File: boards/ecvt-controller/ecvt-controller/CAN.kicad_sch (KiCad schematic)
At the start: 19 parts, among them SW1 SW_SPST, SW2 SW_SPST, U1 TJA1051T-3, U3 MCP2515-xSO, U5 ACT45B-101-2P-TL003, U6 PESD2CAN,215, Y1 Crystal

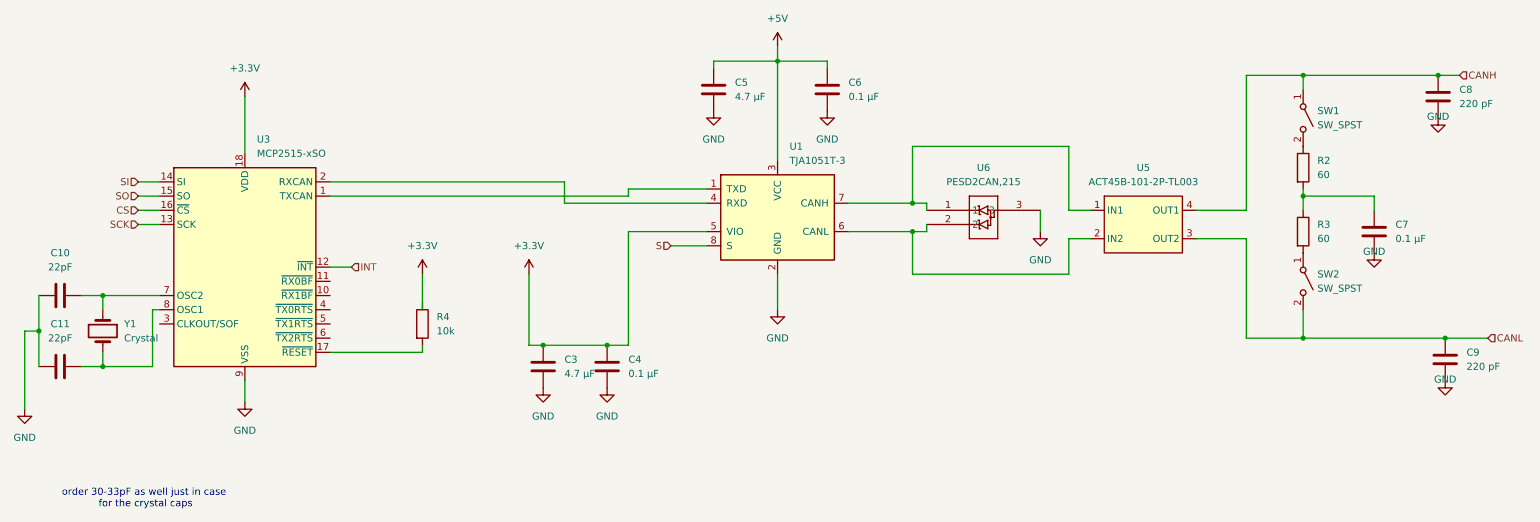
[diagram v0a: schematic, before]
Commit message: components done. RAHHHHH
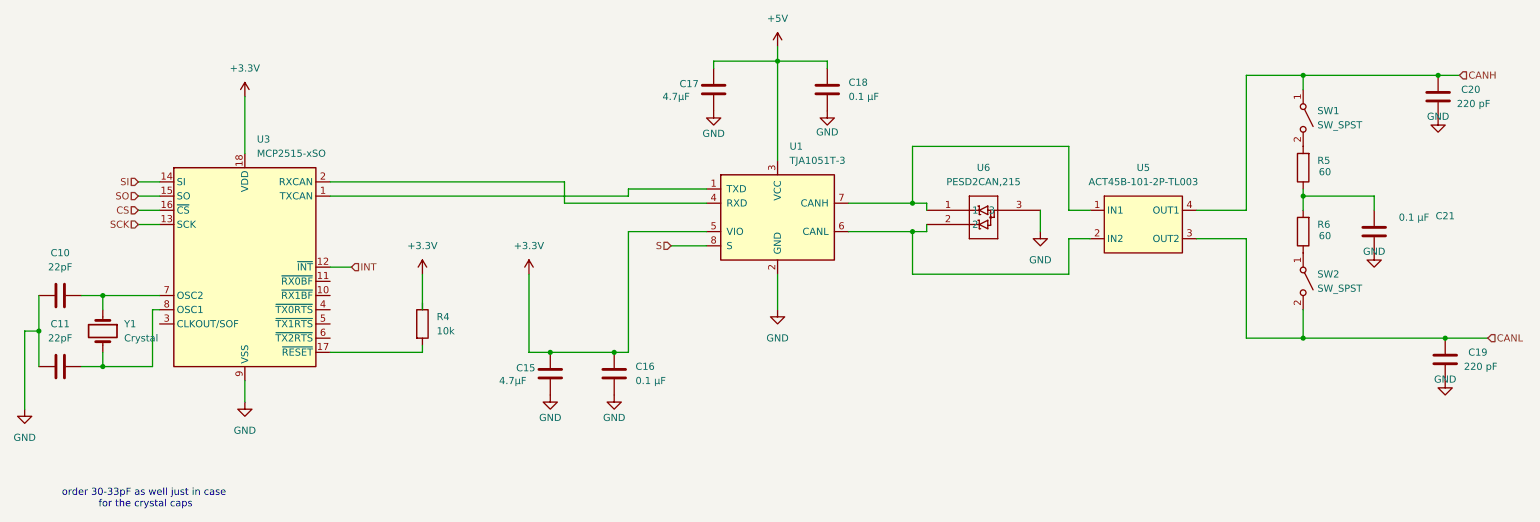
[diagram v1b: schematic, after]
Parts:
- removed C3, C5: 4.7 µF, symbol Device:C
- removed C4, C6, C7: 0.1 µF, symbol Device:C
- removed C8, C9: 220 pF, symbol Device:C
- removed R2, R3: 60, symbol Device:R
- added C15, C17: 4.7µF, Capacitor_SMD:C_0603_1608Metric_Pad1.08x0.95mm_HandSolder, symbol Device:C
- added C16, C18, C21: 0.1 µF, Capacitor_SMD:C_0603_1608Metric_Pad1.08x0.95mm_HandSolder, symbol Device:C
- added C19, C20: 220 pF, Capacitor_SMD:C_0603_1608Metric_Pad1.08x0.95mm_HandSolder, symbol Device:C
- added R5, R6: 60, Resistor_SMD:R_1206_3216Metric_Pad1.30x1.75mm_HandSolder, symbol Device:R
- C10, C11: footprint (none) -> Capacitor_SMD:C_0805_2012Metric_Pad1.18x1.45mm_HandSolder
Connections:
- net +3.3V: now also C15.1, C16.1
- net +5V: now also C17.1, C18.1
- net CANH: now also C20.1
- net CANL: now also C19.1
- net GND: now also C15.2, C16.2, C17.2, C18.2, C19.2, C20.2, C21.1
- net at SW2.1 (A): now also R6.1
- net at SW1.2 (B): now also R5.2
- new net: C21.2, R5.1, R6.2
